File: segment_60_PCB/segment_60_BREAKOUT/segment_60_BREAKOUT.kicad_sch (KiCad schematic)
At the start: 11 parts

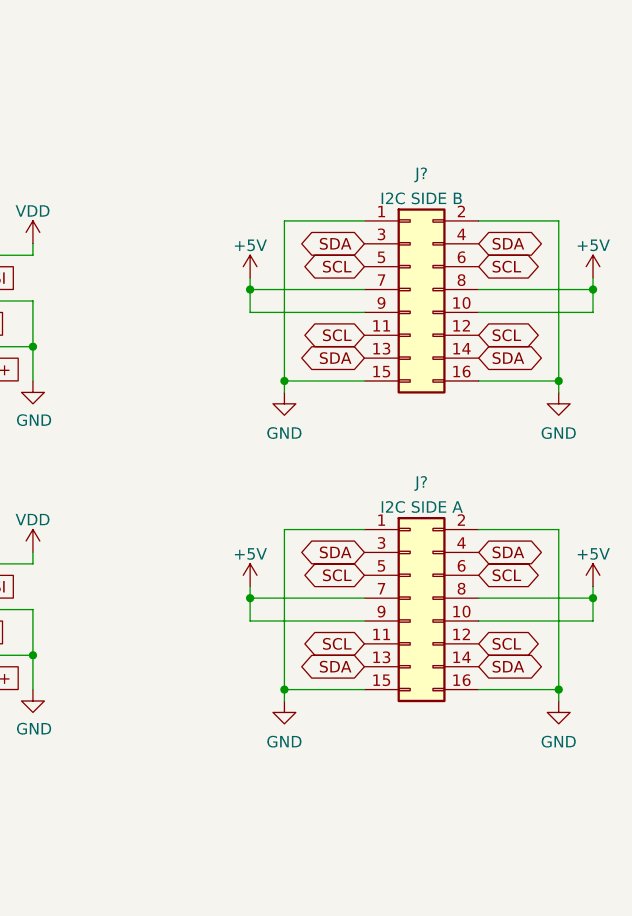
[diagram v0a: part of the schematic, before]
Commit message: Finished silkscreen revisions.
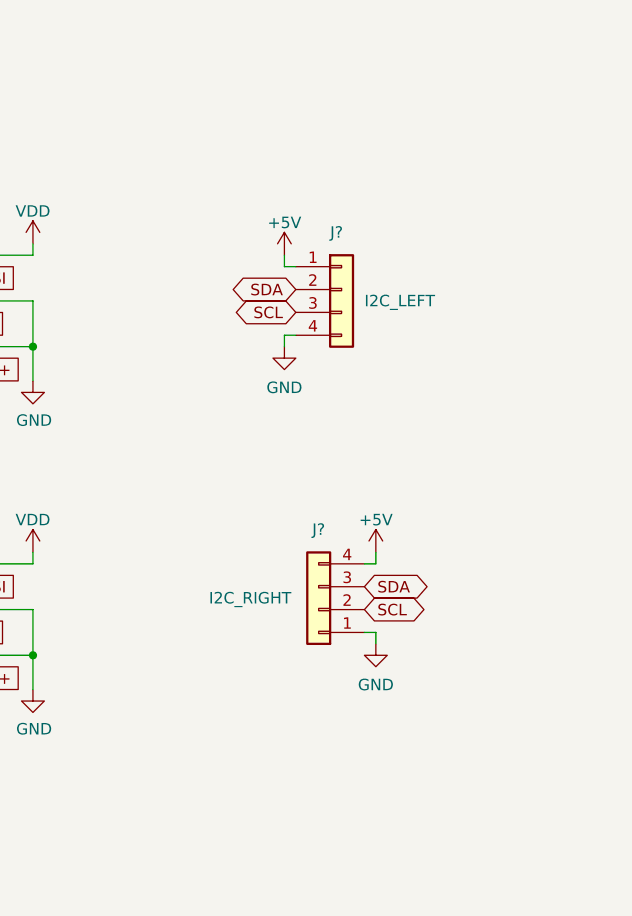
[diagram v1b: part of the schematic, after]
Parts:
- removed J?: I2C SIDE A, symbol Connector_Generic:Conn_02x08_Odd_Even
- removed J?: I2C SIDE B, symbol Connector_Generic:Conn_02x08_Odd_Even
- added J?: I2C_RIGHT, symbol Connector_Generic:Conn_01x04
- added J?: I2C_LEFT, symbol Connector_Generic:Conn_01x04
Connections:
- net +5V: now also J?.1 (Pin_1), J?.4 (Pin_4)
- net GND: now also J?.1 (Pin_1), J?.4 (Pin_4)
- net SCL: now also J?.2 (Pin_2), J?.3 (Pin_3)
- net SDA: now also J?.2 (Pin_2), J?.3 (Pin_3)
